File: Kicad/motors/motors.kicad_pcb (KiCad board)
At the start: 2 copper layers, 80 x 140 mm, 149 parts, among them K100 9V - 1A, K201 MOTOR 1, K202 MOTOR 2, K203 MOTOR 4, K204 MOTOR 3, K301 FRONT, K302 REAR, Q100 DMP2305U, Q101 DMP2305U, Q102 STN790A, Q301 BC846BS, Q302 BC846BS, U100 BQ2057W, U201 L298P, U202 SN74LVC1G19, U203 SN74LVC1G19, U204 L298P, U205 SN74LVC1G19, U206 SN74LVC1G19, U207 LM3480-50, U301 SN74LVC2G17, U302 SN74LVC2G17, U303 LM3480-33

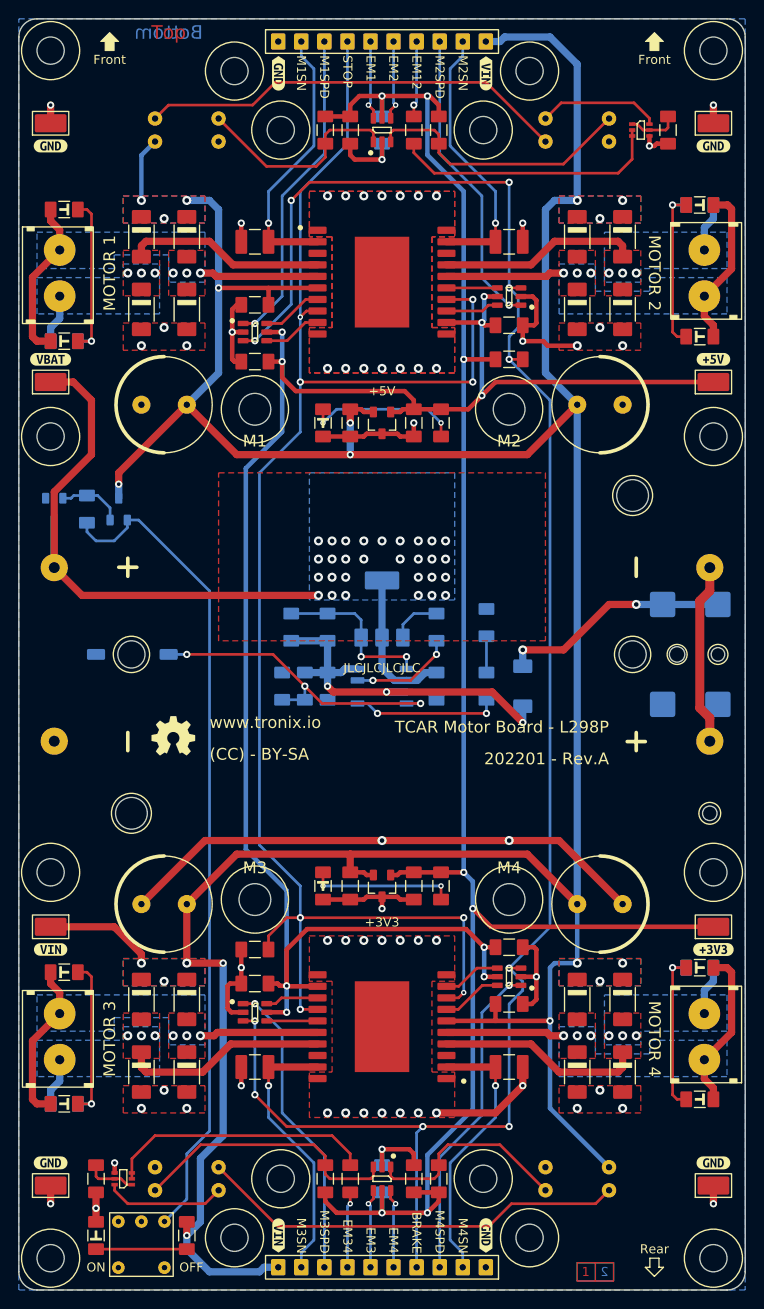
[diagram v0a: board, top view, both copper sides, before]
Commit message: Up
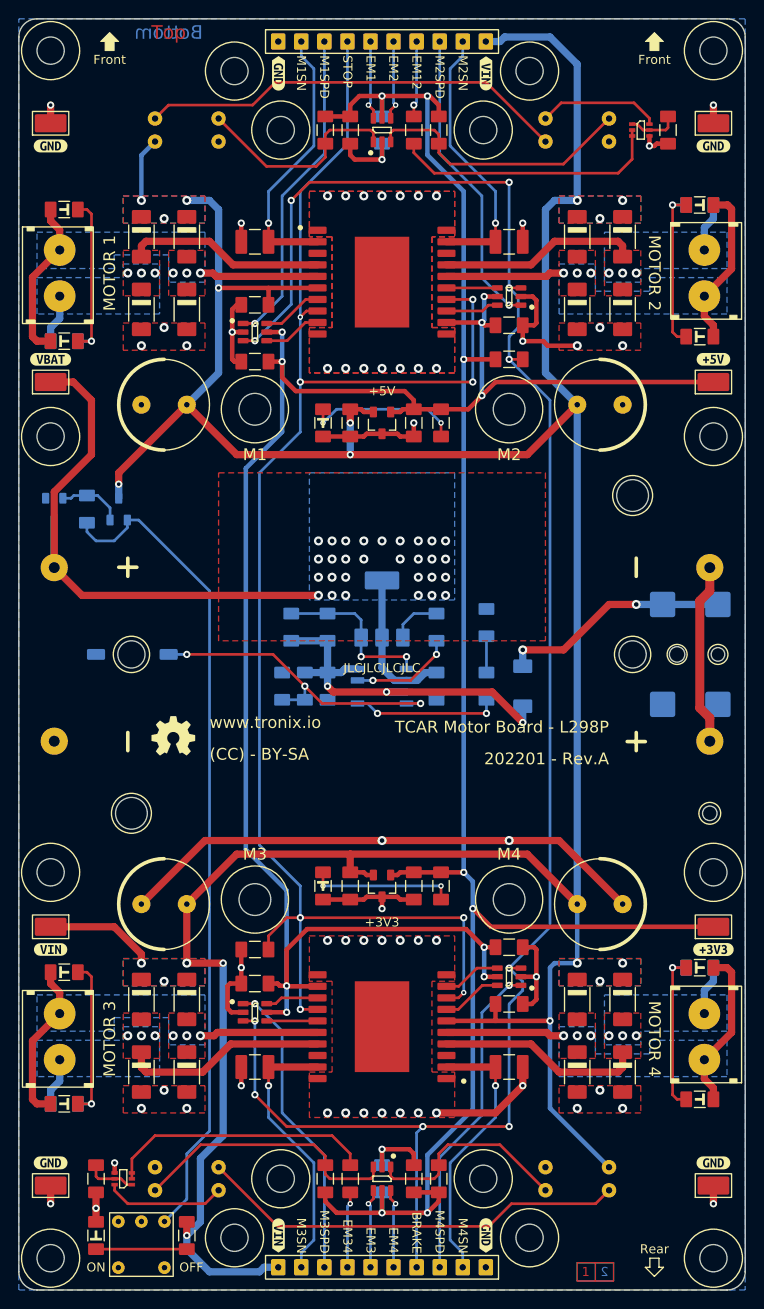
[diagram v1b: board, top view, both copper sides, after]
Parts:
- C203, C204, C207, C208: footprint tronixioZZZ:CAPACITOR-ELECTROLYTIC-RADIAL-100-160-050 -> tronixio:ZZ_CAPACITOR-ELECTROLYTIC-RADIAL-100-160-050
